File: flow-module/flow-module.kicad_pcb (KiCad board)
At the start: 2 copper layers, 49.5 x 35.6 mm, 10 parts, among them P1 TERM_01X02, P3 MOLEX_01X06, P5 TERM_01X02

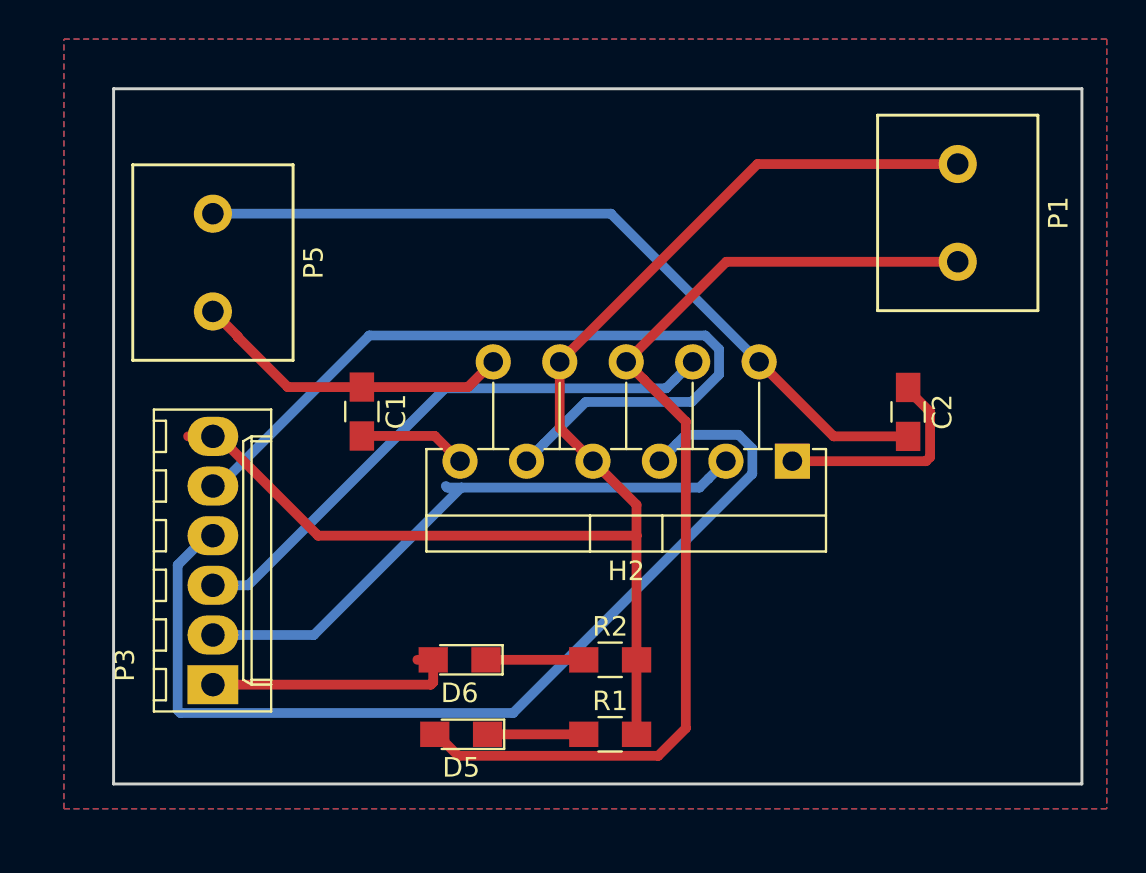
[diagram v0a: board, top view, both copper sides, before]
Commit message: Saved changes
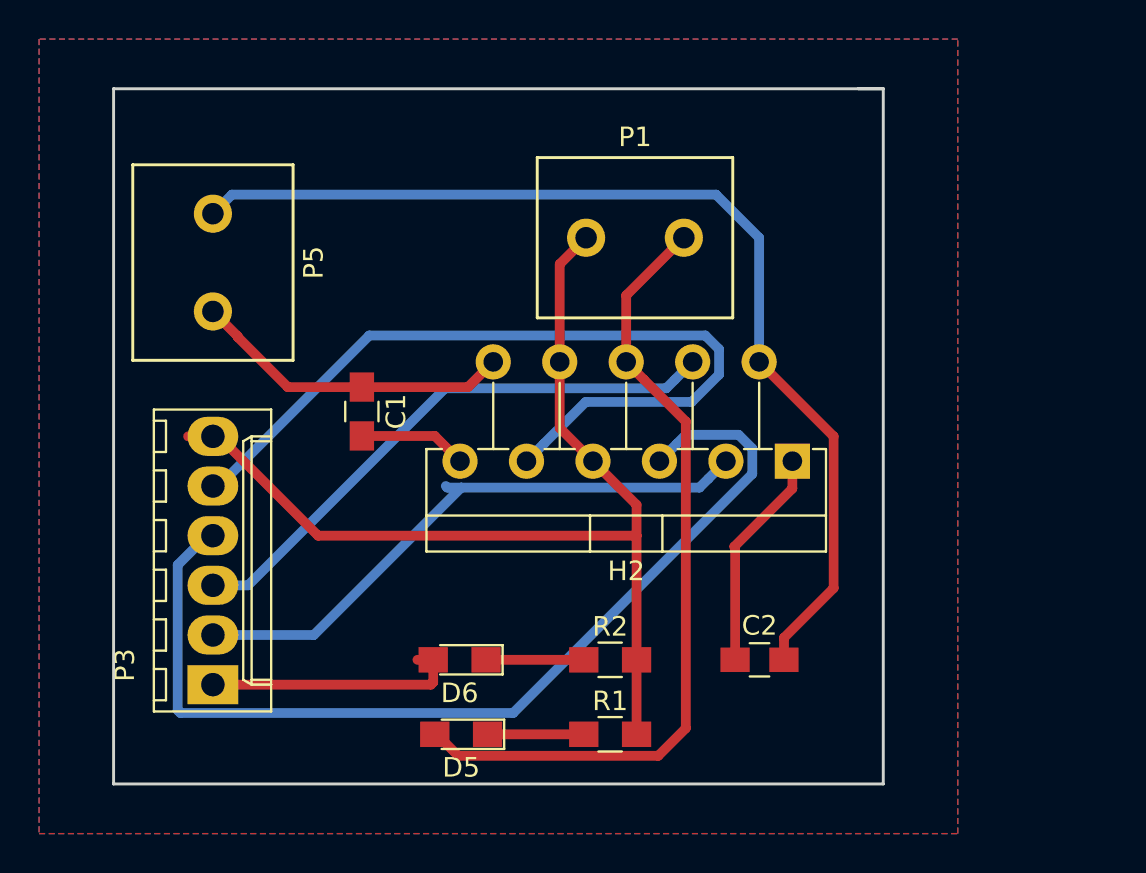
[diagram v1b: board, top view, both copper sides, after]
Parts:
- moved P1 16.6 mm to (96.5, 29.2), turned to 180 degrees
- moved C2 14.8 mm to (102.9, 50.8), turned to 0 degrees
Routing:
- net Earth: track 69.3 -> 51.7 mm
- net Output1: track 40.3 -> 53.5 mm
- net VCC: track 53.0 -> 41.5 mm
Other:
- board size 49.5 x 35.6 mm -> 39.4 x 35.6 mm
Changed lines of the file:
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@@
-(kicad_pcb (version 4) (host pcbnew 4.0.7+dfsg1-1ubuntu2)
+(kicad_pcb (version 20171130) (host pcbnew "(5.0.0-3-g5ebb6b6)")
   (general
-    (links 20)
-    (no_connects 0)
-    (area 67.31 19.05 120.650001 58.420001)
     (thickness 1.6)
-    (drawings 4)
-    (tracks 77)
+    (drawings 6)
+    (tracks 81)
     (zones 0)
     (modules 10)
@@
     (visible_elements 7FFFFFFF)
     (pcbplotparams
-      (layerselection 0x010c0_80000001)
+      (layerselection 0x010c0_ffffffff)
       (usegerberextensions false)
+      (usegerberattributes false)
+      (usegerberadvancedattributes false)
+      (creategerberjobfile false)
       (excludeedgelayer true)
       (linewidth 0.100000)
@@
       (hpglpennumber 1)
       (hpglpenspeed 20)
-      (hpglpendiameter 15)
-      (hpglpenoverlay 2)
+      (hpglpendiameter 15.000000)
       (psnegative false)
       (psa4output false)
@@
       (padsonsilk false)
       (subtractmaskfromsilk false)
-      (outputformat 1)
+      (outputformat 4)
       (mirror false)
       (drillshape 0)
       (scaleselection 1)
-      (outputdirectory "Drill Files/"))
+      (outputdirectory "PDF/"))
   )
   (net 0 "")
@@
   )
   (module ValveTeam:TE_TERM (layer F.Cu)
-    (at 113.03 27.94 90)
-    (fp_text reference P1 (at 0 5.15 90) (layer F.SilkS)
-      (effects (font (size 1 1) (thickness 0.15)))
-    )
-    (fp_text value TERM_01X02 (at -3.81 -5.08 90) (layer F.Fab)
+    (at 96.52 29.21 180)
+    (fp_text reference P1 (at 0 5.15 180) (layer F.SilkS)
+      (effects (font (size 1 1) (thickness 0.15)))
+    )
+    (fp_text value TERM_01X02 (at -3.81 -5.08 180) (layer F.Fab)
       (effects (font (size 1 1) (thickness 0.15)))
     )
@@
     (fp_line (start -5 4.1) (end 5 4.1) (layer F.SilkS) (width 0.15))
     (fp_line (start -5 -4.1) (end -5 4.1) (layer F.SilkS) (width 0.15))
-    (pad 2 thru_hole circle (at 2.5 0 90) (size 1.95 1.95) (drill 1.1) (layers *.Cu *.Mask F.SilkS)
+    (pad 2 thru_hole circle (at 2.5 0 180) (size 1.95 1.95) (drill 1.1) (layers *.Cu *.Mask F.SilkS)
       (net 6 Earth))
-    (pad 1 thru_hole circle (at -2.5 0 90) (size 1.95 1.95) (drill 1.1) (layers *.Cu *.Mask F.SilkS)
+    (pad 1 thru_hole circle (at -2.5 0 180) (size 1.95 1.95) (drill 1.1) (layers *.Cu *.Mask F.SilkS)
       (net 5 VCC))
   )
@@
   )
   (module Capacitors_SMD:C_0805_HandSoldering (layer F.Cu)
-    (at 110.49 38.12 270)
+    (at 102.89 50.8)
     (descr "Capacitor SMD 0805, hand soldering")
     (tags "capacitor 0805")
     (attr smd)
-    (fp_text reference C2 (at 0 -1.75 270) (layer F.SilkS)
-      (effects (font (size 1 1) (thickness 0.15)))
-    )
-    (fp_text value C (at 0 1.75 270) (layer F.Fab)
-      (effects (font (size 1 1) (thickness 0.15)))
-    )
-    (fp_text user %R (at 0 -1.75 270) (layer F.Fab)
+    (fp_text reference C2 (at 0 -1.75) (layer F.SilkS)
+      (effects (font (size 1 1) (thickness 0.15)))
+    )
+    (fp_text value C (at 0 1.75) (layer F.Fab)
+      (effects (font (size 1 1) (thickness 0.15)))
+    )
+    (fp_text user %R (at 0 -1.75) (layer F.Fab)
       (effects (font (size 1 1) (thickness 0.15)))
     )
@@
     (fp_line (start 2.25 0.87) (end 2.25 -0.88) (layer F.CrtYd) (width 0.05))
     (fp_line (start 2.25 0.87) (end -2.25 0.87) (layer F.CrtYd) (width 0.05))
-    (pad 1 smd rect (at -1.25 0 270) (size 1.5 1.25) (layers F.Cu F.Paste F.Mask)
+    (pad 1 smd rect (at -1.25 0) (size 1.5 1.25) (layers F.Cu F.Paste F.Mask)
       (net 3 "Net-(C2-Pad1)"))
-    (pad 2 smd rect (at 1.25 0 270) (size 1.5 1.25) (layers F.Cu F.Paste F.Mask)
+    (pad 2 smd rect (at 1.25 0) (size 1.5 1.25) (layers F.Cu F.Paste F.Mask)
       (net 4 Output1))
     (model Capacitors_SMD.3dshapes/C_0805.wrl
@@
       (net 1 Output2))
   )
-  (gr_line (start 69.85 57.15) (end 119.38 57.15) (angle 90) (layer Edge.Cuts) (width 0.15))
-  (gr_line (start 119.38 57.15) (end 119.38 21.59) (angle 90) (layer Edge.Cuts) (width 0.15))
+  (gr_line (start 109.22 21.59) (end 109.22 57.15) (layer Edge.Cuts) (width 0.15))
+  (gr_line (start 107.95 21.59) (end 109.22 21.59) (layer Edge.Cuts) (width 0.15))
+  (gr_line (start 109.22 21.59) (end 107.95 21.59) (layer Edge.Cuts) (width 0.15))
+  (gr_line (start 69.85 21.59) (end 107.95 21.59) (layer Edge.Cuts) (width 0.15))
+  (gr_line (start 69.85 57.15) (end 109.22 57.15) (angle 90) (layer Edge.Cuts) (width 0.15))
   (gr_line (start 69.85 57.15) (end 69.85 21.59) (angle 90) (layer Edge.Cuts) (width 0.15))
-  (gr_line (start 69.85 21.59) (end 119.38 21.59) (angle 90) (layer Edge.Cuts) (width 0.15))
   (segment (start 82.55 36.85) (end 87.98 36.85) (width 0.5) (layer F.Cu) (net 1))
   (segment (start 87.98 36.85) (end 89.27 35.56) (width 0.5) (layer F.Cu) (net 1))
@@
   (segment (start 82.55 39.35) (end 86.28 39.35) (width 0.5) (layer F.Cu) (net 2))
   (segment (start 86.28 39.35) (end 87.57 40.64) (width 0.5) (layer F.Cu) (net 2))
-  (segment (start 104.57 40.64) (end 111.405002 40.64) (width 0.5) (layer F.Cu) (net 3))
-  (segment (start 111.405002 40.64) (end 111.615 40.430002) (width 0.5) (layer F.Cu) (net 3))
-  (segment (start 111.615 40.430002) (end 111.615 38.12) (width 0.5) (layer F.Cu) (net 3))
-  (segment (start 111.615 38.12) (end 110.49 36.995) (width 0.5) (layer F.Cu) (net 3))
-  (segment (start 110.49 36.995) (end 110.49 36.87) (width 0.5) (layer F.Cu) (net 3))
-  (segment (start 106.68 39.37) (end 110.49 39.37) (width 0.5) (layer F.Cu) (net 4))
+  (segment (start 101.765 50.8) (end 101.64 50.8) (width 0.5) (layer F.Cu) (net 3))
+  (segment (start 104.57 42.04) (end 101.6 45.01) (width 0.5) (layer F.Cu) (net 3))
+  (segment (start 104.57 40.64) (end 104.57 42.04) (width 0.5) (layer F.Cu) (net 3))
+  (segment (start 101.64 45.05) (end 101.64 50.8) (width 0.5) (layer F.Cu) (net 3))
+  (segment (start 101.6 45.01) (end 101.64 45.05) (width 0.5) (layer F.Cu) (net 3))
   (segment (start 102.87 35.56) (end 106.68 39.37) (width 0.5) (layer F.Cu) (net 4))
-  (segment (start 74.93 27.98) (end 95.29 27.98) (width 0.5) (layer B.Cu) (net 4))
-  (segment (start 95.29 27.98) (end 102.87 35.56) (width 0.5) (layer B.Cu) (net 4))
-  (segment (start 96.07 35.56) (end 101.19 30.44) (width 0.5) (layer F.Cu) (net 5))
-  (segment (start 101.19 30.44) (end 113.03 30.44) (width 0.5) (layer F.Cu) (net 5))
+  (segment (start 102.87 35.56) (end 102.87 29.21) (width 0.5) (layer B.Cu) (net 4))
+  (segment (start 75.904999 27.005001) (end 74.93 27.98) (width 0.5) (layer B.Cu) (net 4))
+  (segment (start 100.665001 27.005001) (end 75.904999 27.005001) (width 0.5) (layer B.Cu) (net 4))
+  (segment (start 102.87 29.21) (end 100.665001 27.005001) (width 0.5) (layer B.Cu) (net 4))
+  (segment (start 104.14 49.675) (end 106.68 47.135) (width 0.5) (layer F.Cu) (net 4))
+  (segment (start 104.14 50.8) (end 104.14 49.675) (width 0.5) (layer F.Cu) (net 4))
+  (segment (start 106.68 47.135) (end 106.68 39.37) (width 0.5) (layer F.Cu) (net 4))
   (segment (start 86.28 54.61) (end 86.38 54.61) (width 0.5) (layer F.Cu) (net 5))
   (segment (start 86.38 54.61) (end 87.480001 55.710001) (width 0.5) (layer F.Cu) (net 5))
@@
   (segment (start 99.120001 38.610001) (end 96.969999 36.459999) (width 0.5) (layer F.Cu) (net 5))
   (segment (start 96.969999 36.459999) (end 96.07 35.56) (width 0.5) (layer F.Cu) (net 5))
-  (segment (start 92.67 35.56) (end 102.79 25.44) (width 0.5) (layer F.Cu) (net 6))
-  (segment (start 102.79 25.44) (end 113.03 25.44) (width 0.5) (layer F.Cu) (net 6))
+  (segment (start 96.07 32.16) (end 99.02 29.21) (width 0.5) (layer F.Cu) (net 5))
+  (segment (start 96.07 35.56) (end 96.07 32.16) (width 0.5) (layer F.Cu) (net 5))
   (segment (start 96.6 50.8) (end 96.6 44.45) (width 0.5) (layer F.Cu) (net 6))
   (segment (start 74.93 39.37) (end 75.23 39.37) (width 0.5) (layer F.Cu) (net 6))
@@
   (segment (start 96.6 42.87) (end 94.37 40.64) (width 0.5) (layer F.Cu) (net 6))
   (segment (start 73.96 39.37) (end 73.66 39.37) (width 0.5) (layer F.Cu) (net 6))
+  (segment (start 92.67 30.56) (end 94.02 29.21) (width 0.5) (layer F.Cu) (net 6))
+  (segment (start 92.67 35.56) (end 92.67 30.56) (width 0.5) (layer F.Cu) (net 6))
   (segment (start 88.98 54.61) (end 93.9 54.61) (width 0.5) (layer F.Cu) (net 7))
   (segment (start 88.9 50.8) (end 89 50.8) (width 0.5) (layer F.Cu) (net 8))
@@
     (polygon
       (pts
-        (xy 67.31 19.05) (xy 120.65 19.05) (xy 120.65 58.42) (xy 67.31 58.42)
+        (xy 66.04 19.05) (xy 66.04 59.69) (xy 113.03 59.69) (xy 113.03 19.05)
       )
     )
@@
     (polygon
       (pts
-        (xy 67.31 19.05) (xy 120.65 19.05) (xy 120.65 58.42) (xy 67.31 58.42)
+        (xy 66.04 19.05) (xy 66.04 59.69) (xy 113.03 59.69) (xy 113.03 19.05)
       )
     )
